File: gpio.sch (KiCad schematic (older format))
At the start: 3 parts, among them J1 DF40C-100DP-0.4V(51), J2 DF40C-100DP-0.4V(51), U1 LFE5U-85F-6BG381C

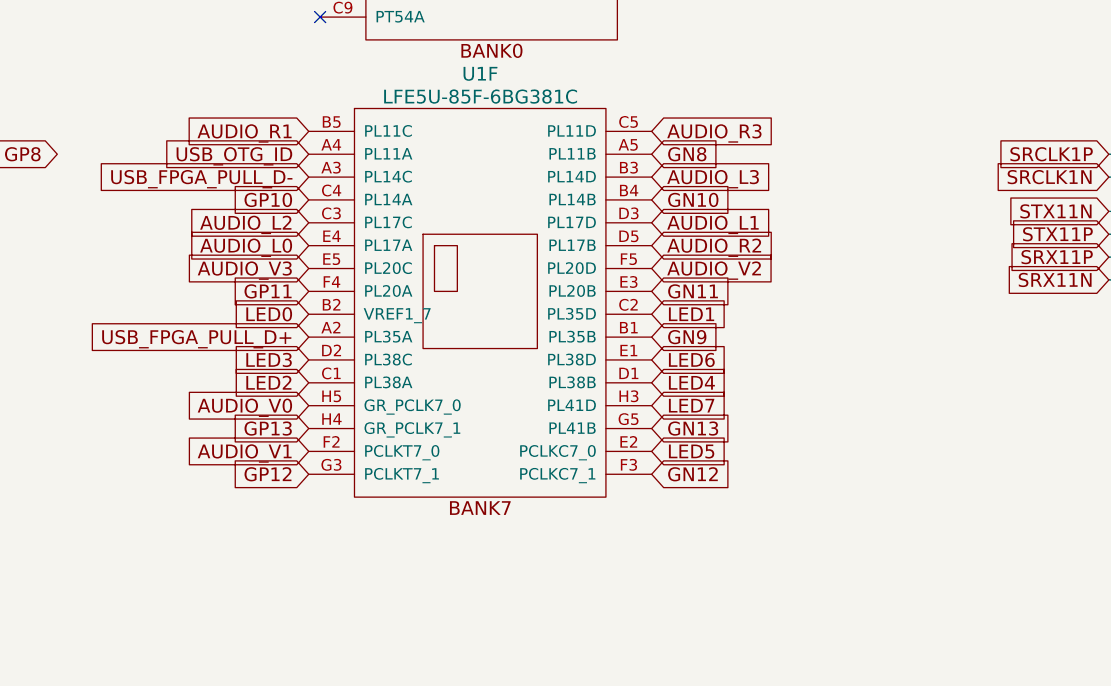
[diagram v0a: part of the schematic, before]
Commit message: Adding buttons
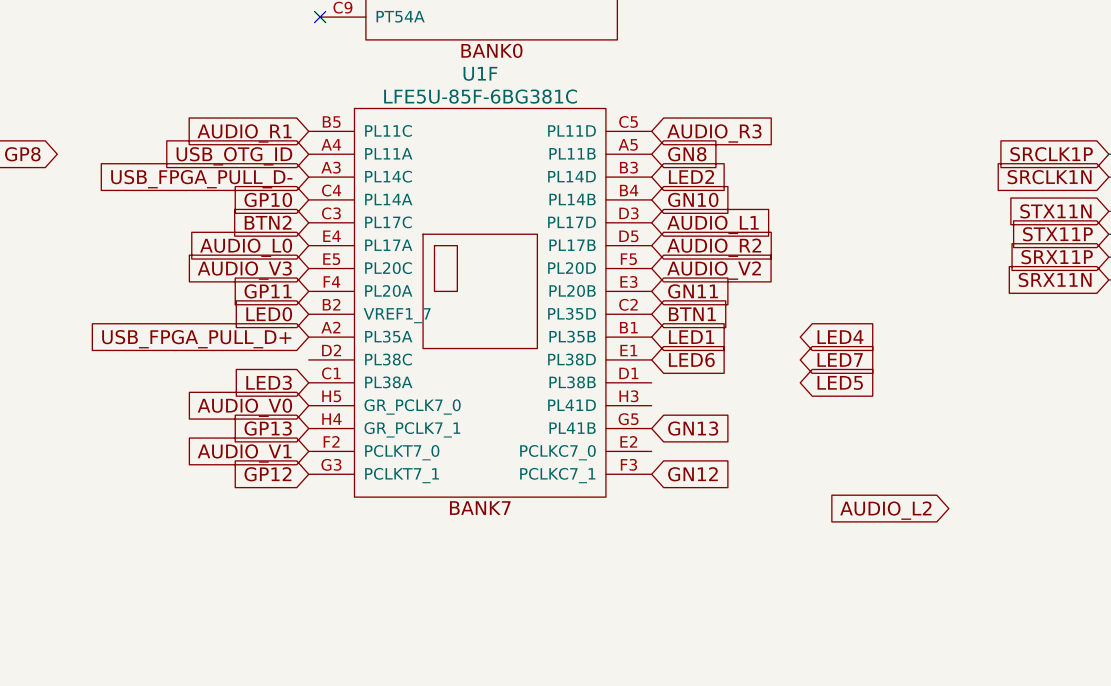
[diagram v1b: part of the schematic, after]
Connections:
- net AUDIO_L3 is gone; now on net LED2: U1.B3 (PL14D)
- net AUDIO_L2: no longer U1.C3 (PL17C)
- net GN9: no longer U1.B1 (PL35B)
- net LED1: now also U1.B1 (PL35B); no longer U1.C2 (PL35D)
- net LED2: no longer U1.C1 (PL38A)
- net LED3: now also U1.C1 (PL38A); no longer U1.D2 (PL38C)
- net LED4: no longer U1.D1 (PL38B)
- net LED5: no longer U1.E2 (PCLKC7_0)
- net LED7: no longer U1.H3 (PL41D)
- new net BTN1: U1.C2 (PL35D)
- new net BTN2: U1.C3 (PL17C)
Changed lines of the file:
@@
 Text GLabel 1050 3300 0    60   Input ~ 0
 GP11
-Text GLabel 2550 3500 2    60   Input ~ 0
-GN9
+Text GLabel 2550 3400 2    60   Input ~ 0
+BTN1
 Text GLabel -600 3450 0    60   Input ~ 0
 GP9
@@
 Text GLabel 2550 3000 2    60   Input ~ 0
 AUDIO_L1
+Text GLabel 3850 4250 0    60   Input ~ 0
+AUDIO_L2
 Text GLabel 1050 3000 0    60   Input ~ 0
-AUDIO_L2
-Text GLabel 2550 2800 2    60   Input ~ 0
-AUDIO_L3
+BTN2
 Text GLabel -500 3300 0    60   Input ~ 0
 AUDIO_R0
@@
 Text GLabel 1050 3400 0    60   Input ~ 0
 LED0
-Text GLabel 2550 4000 2    60   Input ~ 0
+Text GLabel 3200 3700 2    60   Input ~ 0
 LED5
+Text GLabel 2550 2800 2    60   Input ~ 0
+LED2
 Text GLabel 1050 3700 0    60   Input ~ 0
-LED2
-Text GLabel 1050 3600 0    60   Input ~ 0
 LED3
-Text GLabel 2550 3700 2    60   Input ~ 0
+Text GLabel 3200 3500 2    60   Input ~ 0
 LED4
-Text GLabel 2550 3400 2    60   Input ~ 0
-LED1
 Text GLabel 2550 3600 2    60   Input ~ 0
 LED6
-Text GLabel 2550 3800 2    60   Input ~ 0
+Text GLabel 3200 3600 2    60   Input ~ 0
 LED7
 Text Notes 950  7550 0    60   ~ 0
@@
 CM4_3.3V
 $Comp
-L power:+3V3 #PWR?
+L power:+3V3 #PWR0111
 U 1 1 61646D74
 P 5200 4900
-F 0 "#PWR?" H 5200 4750 50  0001 C CNN
+F 0 "#PWR0111" H 5200 4750 50  0001 C CNN
 F 1 "+3V3" H 5200 5040 50  0000 C CNN
 F 2 "" H 5200 4900 50  0000 C CNN
@@
 Text Notes 5050 5600 1    60   ~ 0
 CM4 needs to provide 3.3V to CM4 IO board
+Text GLabel 2550 3500 2    60   Input ~ 0
+LED1
 $EndSCHEMATC
